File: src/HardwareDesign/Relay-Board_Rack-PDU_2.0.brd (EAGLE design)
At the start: 156.1 x 120 mm, 215 parts, among them IC1 MP2315GJ-Z, IC10 HLW8032, IC11 HLW8032, IC12 HLW8032, IC14 HLW8032, IC16 HLW8032, IC2 MP2315S, IC3 ULN2803A, IC4 MCP23017-E/ML, IC5 BA50BC0FP-E2, IC6 HLW8032, IC7 HLW8032, IC8 HLW8032, IC9 SN74HC151PWR, J1 FPC20-H, K1 G2RL-1A-E_DC12, K2 G2RL-1A-E_DC12, K3 G2RL-1A-E_DC12, K4 G2RL-1A-E_DC12, K5 G2RL-1A-E_DC12, K6 G2RL-1A-E_DC12, K7 G2RL-1A-E_DC12, K8 G2RL-1A-E_DC12, SW3 TP

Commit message: add datasheets for Rev2.0
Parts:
- AC/DC1: value (none) -> IRM_10_12
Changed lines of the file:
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@@
 <drawing>
 <settings>
-<setting alwaysvectorfont="yes"/>
+<setting alwaysvectorfont="no"/>
 <setting verticaltext="up"/>
 </settings>
@@
 <attribute name="VALUE" x="153.345" y="-50.075" size="1.27" layer="27" rot="R90"/>
 </element>
-<element name="AC/DC1" library="ds_trafo" package="IRM_10_12" package3d_urn="urn:adsk.eagle:package:47075710/2" value="" x="54.5" y="59.3" smashed="yes">
+<element name="AC/DC1" library="ds_trafo" package="IRM_10_12" package3d_urn="urn:adsk.eagle:package:47075710/2" value="IRM_10_12" x="54.5" y="59.3" smashed="yes">
 <attribute name="NAME" x="32" y="46.02" size="1.27" layer="25"/>
 <attribute name="VALUE" x="31.4" y="46.62" size="1.27" layer="27" align="top-left"/>

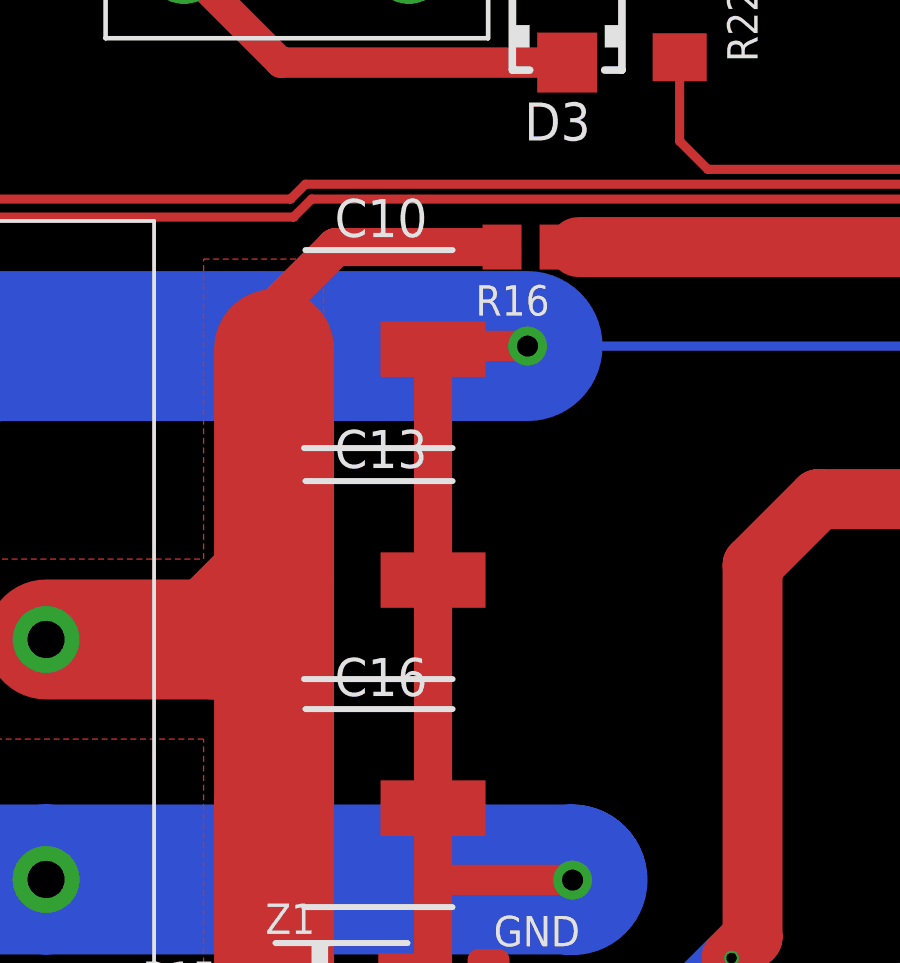
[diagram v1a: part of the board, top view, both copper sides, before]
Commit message: update repo to Rev2.0
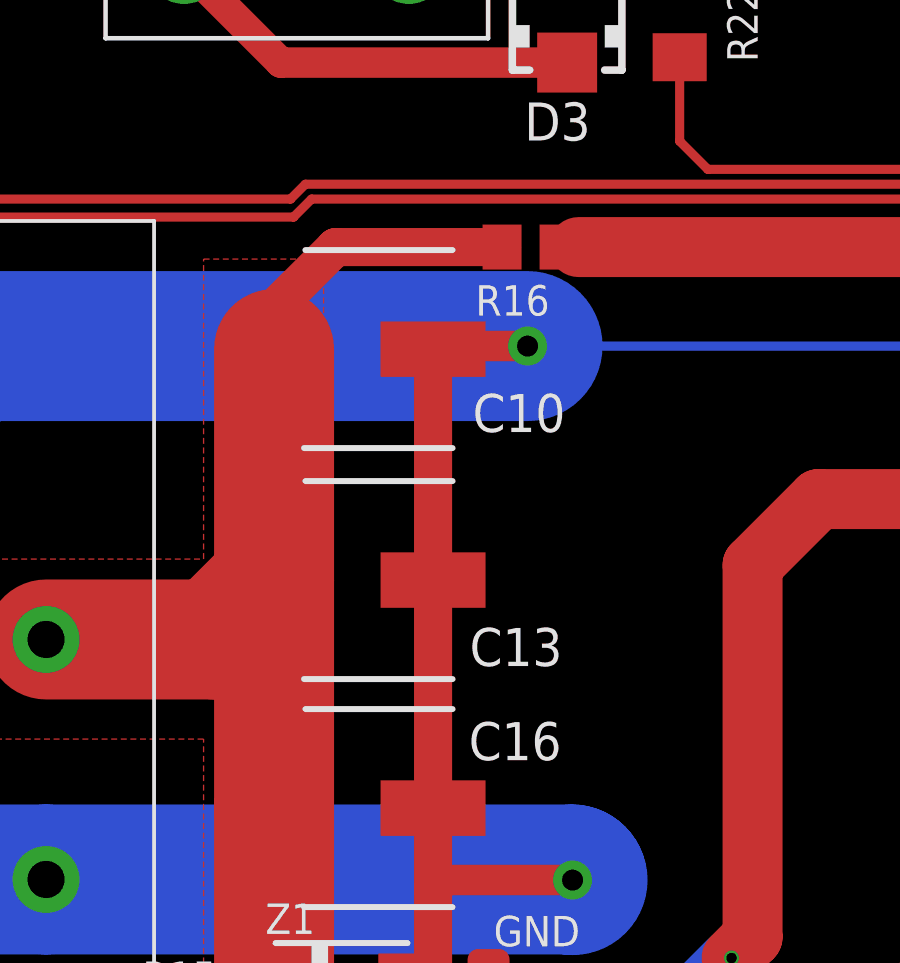
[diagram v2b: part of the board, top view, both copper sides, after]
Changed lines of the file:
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@@
 <wire x1="-1" y1="3.41420625" x2="2.41420625" y2="0" width="0" layer="20" curve="90"/>
 <circle x="3" y="4" radius="3" width="1" layer="29"/>
-<circle x="141" y="4" radius="3" width="1" layer="29"/>
 <circle x="3" y="115.9" radius="2.828425" width="1" layer="29"/>
 <text x="153.98" y="8.39" size="1.4224" layer="25" font="vector" ratio="13" rot="R90">github.com/DvidMakesThings/HW_10-In-Rack_PDU
@@
 </element>
 <element name="C10" library="ds_passive" package="100UF-16V" package3d_urn="urn:adsk.eagle:package:46684204/2" value="100uF" x="84" y="69" smashed="yes">
-<attribute name="NAME" x="84.9144" y="73.3688" size="1.27" layer="25" align="center"/>
+<attribute name="NAME" x="89.5144" y="66.8688" size="1.27" layer="25" align="center"/>
 <attribute name="VALUE" x="84.4572" y="64.6566" size="1.27" layer="27" align="center"/>
 </element>
 <element name="C13" library="ds_passive" package="100UF-16V" package3d_urn="urn:adsk.eagle:package:46684204/2" value="100uF" x="84" y="61.3" smashed="yes">
-<attribute name="NAME" x="84.9144" y="65.6688" size="1.27" layer="25" align="center"/>
+<attribute name="NAME" x="89.4144" y="59.0688" size="1.27" layer="25" align="center"/>
 <attribute name="VALUE" x="84.4572" y="56.9566" size="1.27" layer="27" align="center"/>
 </element>
 <element name="C16" library="ds_passive" package="100UF-16V" package3d_urn="urn:adsk.eagle:package:46684204/2" value="100uF" x="84" y="53.7" smashed="yes">
-<attribute name="NAME" x="84.9144" y="58.0688" size="1.27" layer="25" align="center"/>
+<attribute name="NAME" x="89.3856" y="55.9312" size="1.27" layer="25" rot="R180" align="center"/>
 <attribute name="VALUE" x="84.4572" y="49.3566" size="1.27" layer="27" align="center"/>
 </element>
